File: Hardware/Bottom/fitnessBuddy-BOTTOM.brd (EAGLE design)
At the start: 33 x 33 mm, 47 parts, among them U4 PCF8523

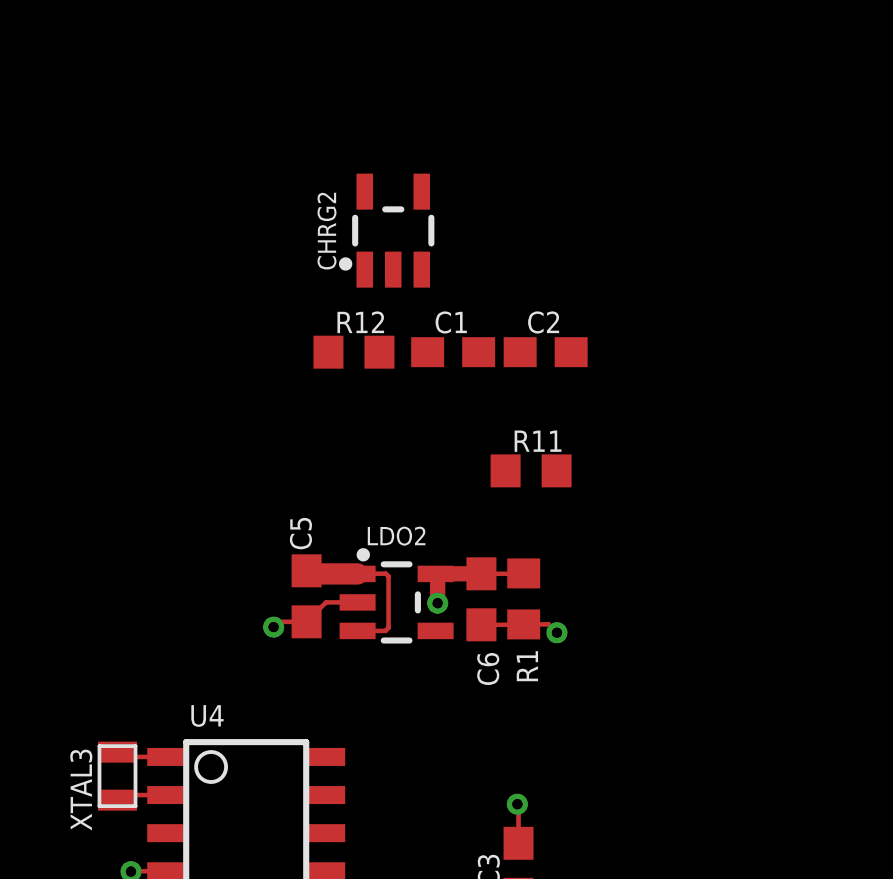
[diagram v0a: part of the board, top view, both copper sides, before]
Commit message: Reorganized top and bottom boards, went back and rerouted some of top board (basically did take 005 and take 006)
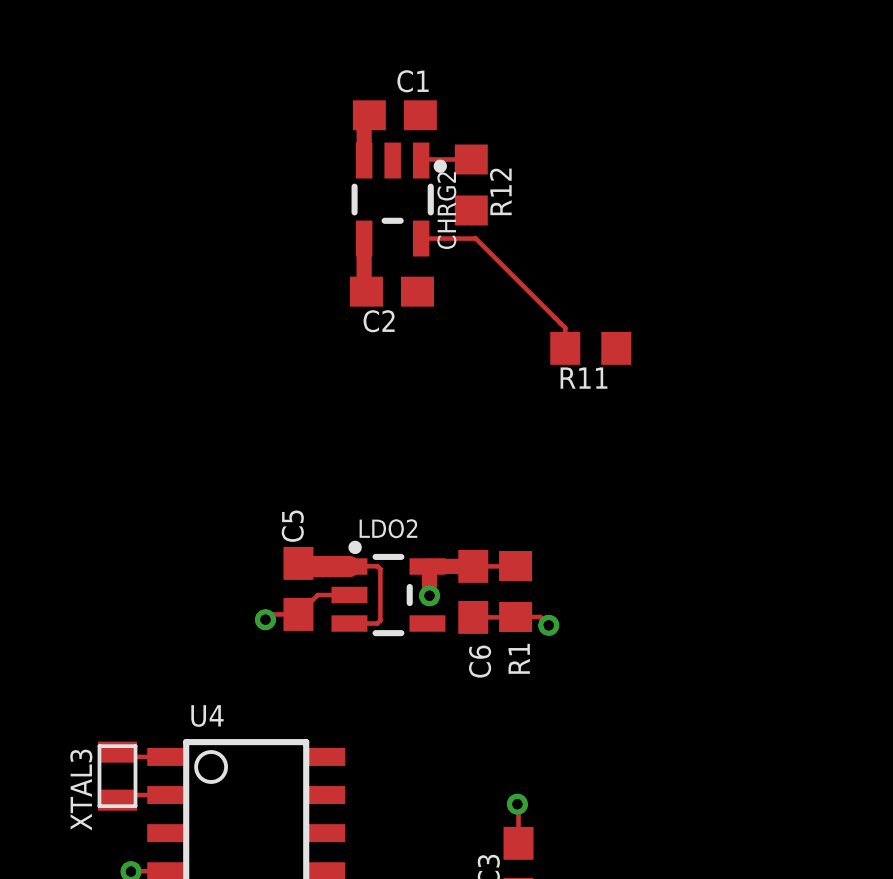
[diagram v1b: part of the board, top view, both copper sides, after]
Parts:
- moved C1 8.13 mm to (-19.3, 42.2)
- moved R12 6.81 mm to (-16.8, 39.9), turned to 270 degrees
- moved C2 5.51 mm to (-19.4, 36.3), turned to 180 degrees
- moved R11 4.54 mm to (-12.8, 34.4), turned to 180 degrees
- moved CHRG2 1.04 mm to (-19.4, 39.4), turned to 180 degrees
- moved C6 0.37 mm to (-16.7, 26.3)
- moved LDO2 0.37 mm to (-19.5, 26.2)
- moved C5 0.37 mm to (-22.5, 26.4)
- moved R1 0.37 mm to (-15.3, 26.3)
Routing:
- net N$4: track 0.00 -> 6.72 mm
- net VIN: track 5.60 -> 7.40 mm
- net D27/CHRG.STATUS: track 0.00 -> 1.69 mm
- net VLIPO: track 0.00 -> 1.58 mm
